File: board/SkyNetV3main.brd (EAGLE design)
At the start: 160 x 100 mm, 61 parts, among them IC1 HC_05, IC2 RF4463PRO, IC3 LPC1768, IC4 BCX17, IC5 TPS63001, IC6 MCP73871-2CCI/ML, Q1 32.768KHz, Q2 12MHz, Q3 IRLM6402, Q4 BSS138, X1 BAT

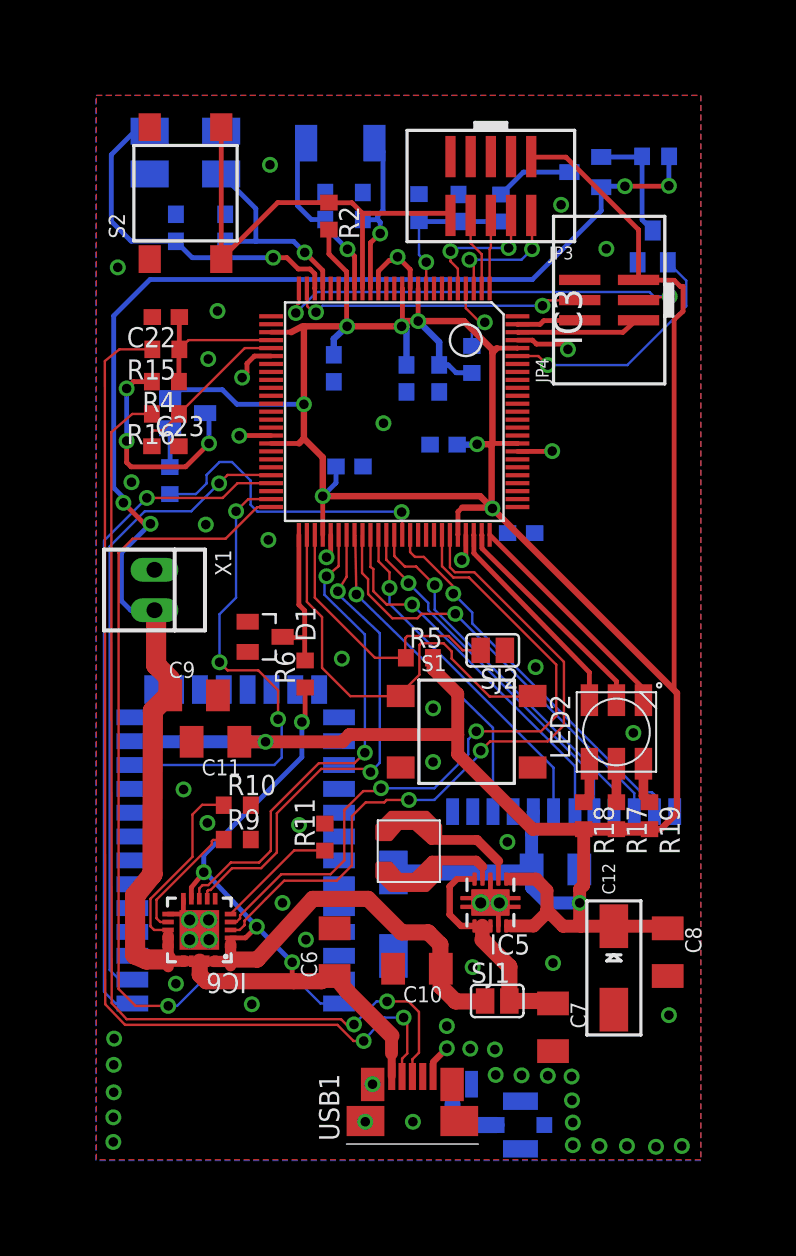
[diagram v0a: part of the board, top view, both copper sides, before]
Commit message: layout improvements
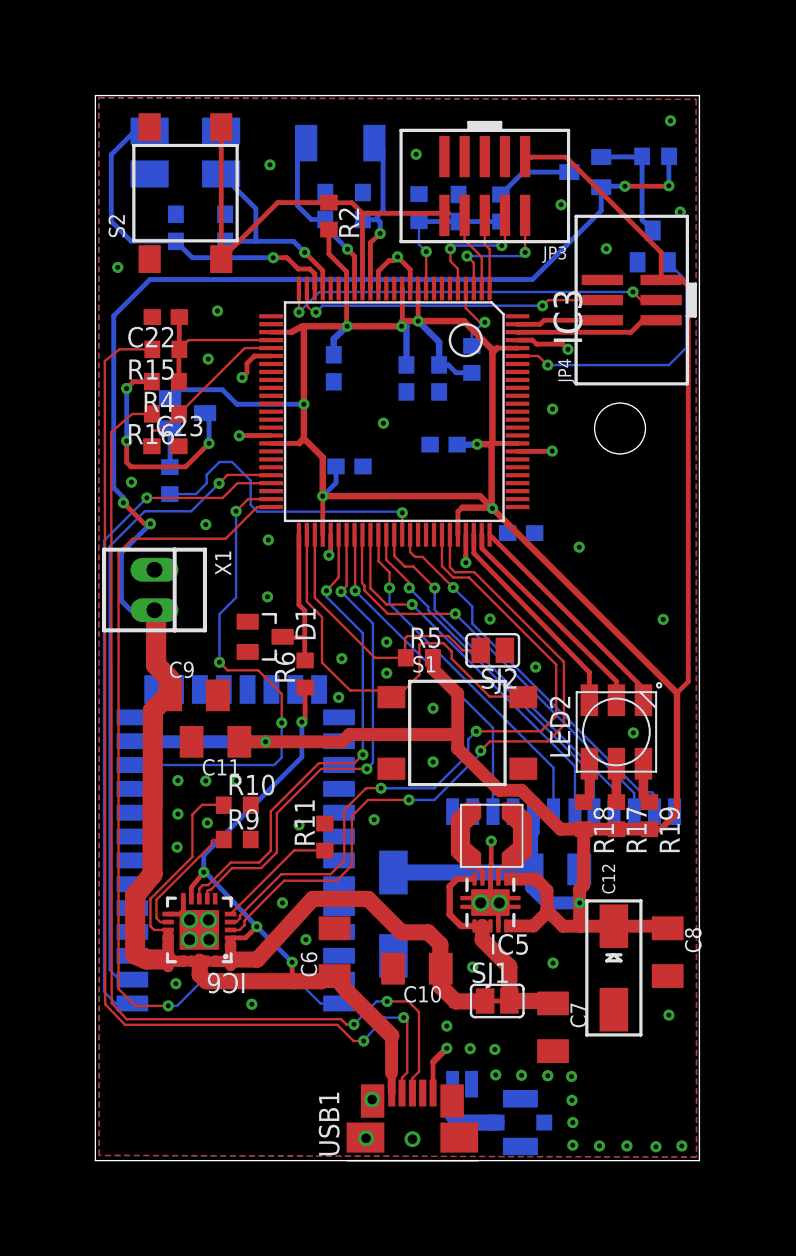
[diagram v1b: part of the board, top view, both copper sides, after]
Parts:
- moved L1 5.56 mm to (114.2, 38.7), turned to 0 degrees
- moved JP4 1.42 mm to (123.0, 72.2)
- moved USB1 1.04 mm to (109.2, 19.5)
- moved S1 0.59 mm to (112.0, 45.0)
- moved JP3 0.38 mm to (113.7, 79.4)
- moved U$1 0.15 mm to (116.0, 20.5)
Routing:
- net GND: track 26.9 -> 31.9 mm, vias 62 -> 73
- net SDA-EXT: track 30.0 -> 25.0 mm
- net L2: track 7.72 -> 3.36 mm
- net +5V: track 45.8 -> 49.1 mm
- net L1: track 6.08 -> 3.24 mm
- net N$1: track 0.00 -> 1.65 mm
- net AD-PWR: track 15.6 -> 17.2 mm
- net TX: track 7.90 -> 9.34 mm
- net RX: track 4.01 -> 5.45 mm
- net SCL-EXT: track 18.7 -> 20.2 mm
- net INPUT: track 27.0 -> 28.3 mm
- net USB-D-_IN: track 63.9 -> 65.0 mm
- net USB-D+_IN: track 68.1 -> 69.1 mm
- net CHG-S2: track 32.0 -> 31.0 mm
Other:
- outline, holes or cut-outs redrawn
